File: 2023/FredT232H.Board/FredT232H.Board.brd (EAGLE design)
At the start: 88 x 77 mm, 17 parts

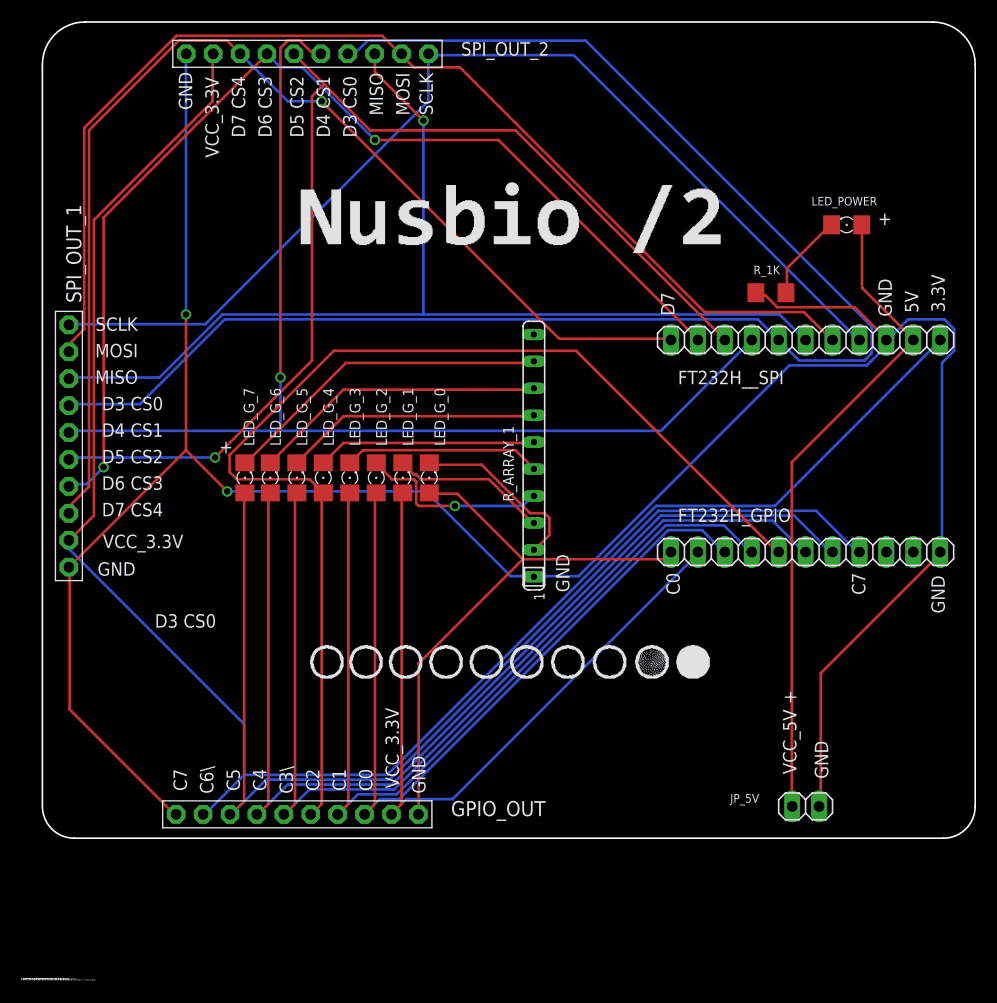
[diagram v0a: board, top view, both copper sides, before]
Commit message: Board 2023 fix first bug
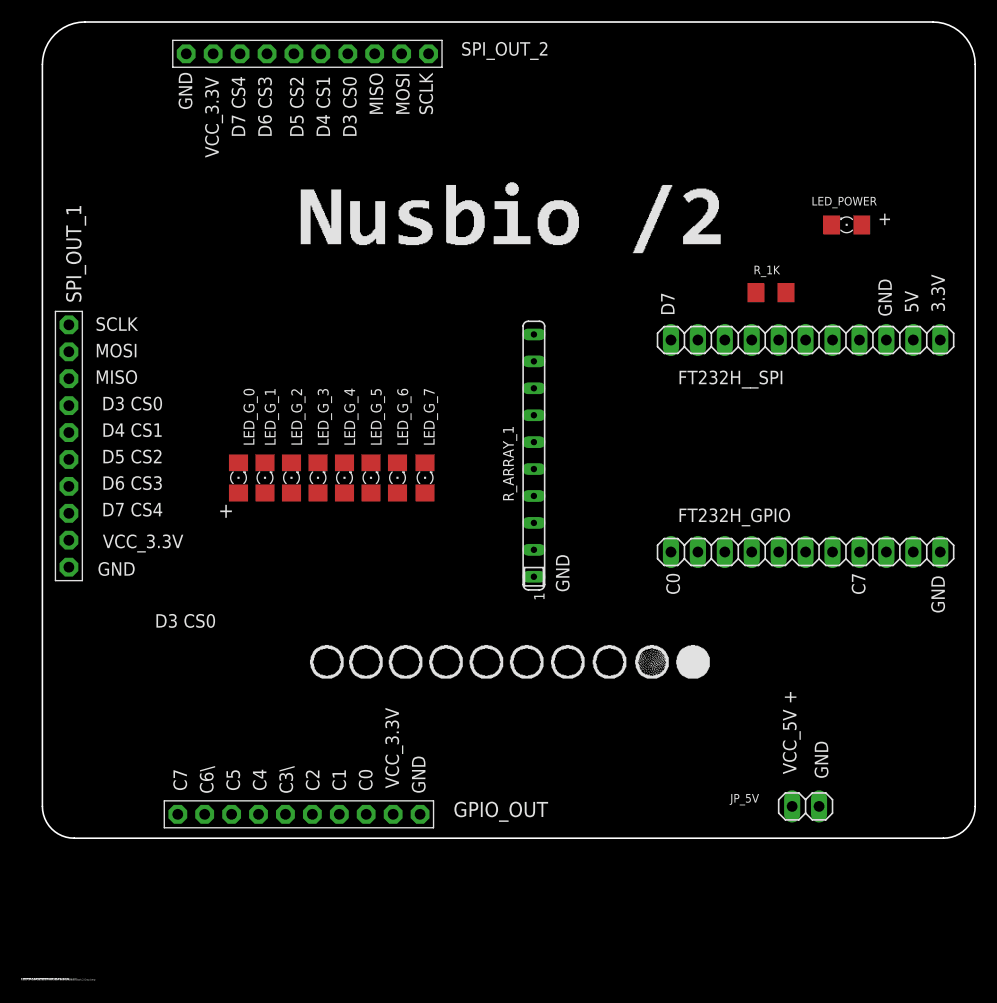
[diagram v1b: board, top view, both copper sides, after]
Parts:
- moved LED_G_0 18.0 mm to (20.5, 47.0)
- moved LED_G_7 17.0 mm to (38.1, 47.0)
- moved LED_G_1 13.0 mm to (23.0, 47.0)
- moved LED_G_6 12.0 mm to (35.5, 47.0)
- moved LED_G_2 8.00 mm to (25.5, 47.0)
- moved LED_G_5 7.00 mm to (33.0, 47.0)
- moved LED_G_3 3.00 mm to (28.0, 47.0)
- moved LED_G_4 2.00 mm to (30.5, 47.0)
- moved GPIO_OUT 0.15 mm to (26.2, 15.3), turned to 180 degrees
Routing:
- net GND: track 233.4 -> 0.00 mm, vias 2 -> 0
- net VCC_33: track 168.6 -> 0.00 mm
- net D3_CS0: track 144.7 -> 0.00 mm
- net D4_CS1: track 108.8 -> 0.00 mm, vias 1 -> 0
- net D1_MOSI: track 107.8 -> 0.00 mm
- net D7_CS4: track 107.1 -> 0.00 mm, vias 1 -> 0
- net C4: track 105.8 -> 0.00 mm
- net D5_CS2: track 105.2 -> 0.00 mm, vias 1 -> 0
- net C7: track 103.8 -> 0.00 mm
- net D6_CS3: track 101.3 -> 0.00 mm, vias 2 -> 0
- net D2_MISO: track 99.5 -> 0.00 mm, vias 1 -> 0
- net D0_SCLK: track 98.9 -> 0.00 mm
- net C6: track 98.3 -> 0.00 mm
- net C5: track 92.8 -> 0.00 mm
- net C3: track 82.2 -> 0.00 mm
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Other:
- board text added: "PCBv2 - 2023.03"
- board text removed: "PCBv1 - 2023.02"
